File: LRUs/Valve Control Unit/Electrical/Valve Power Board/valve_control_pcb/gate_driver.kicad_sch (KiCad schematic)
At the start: 10 parts, among them U14 UCC27524D, U15 UCC27524D

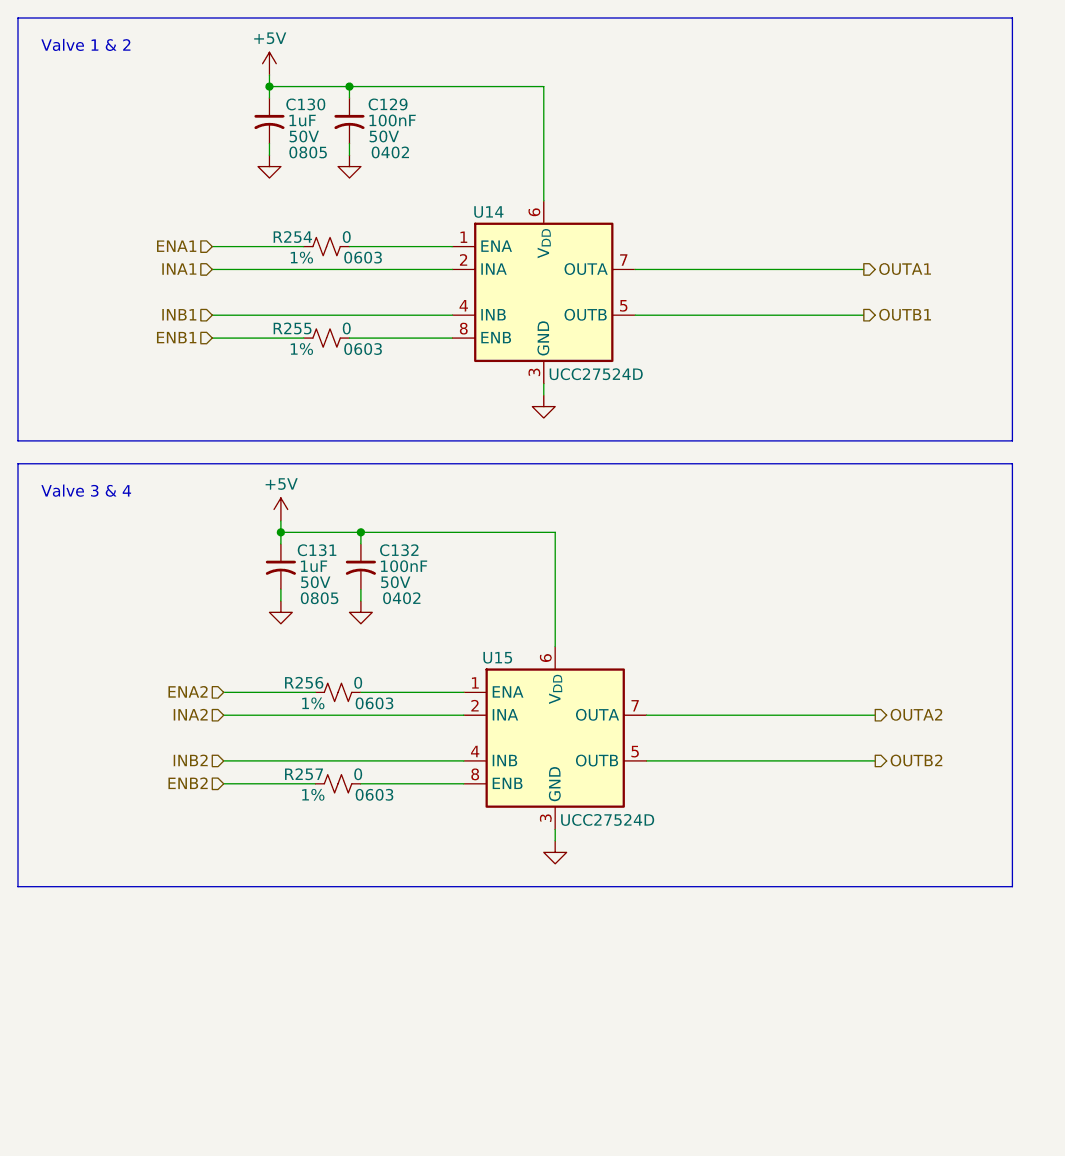
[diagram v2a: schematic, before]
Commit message: Small updates
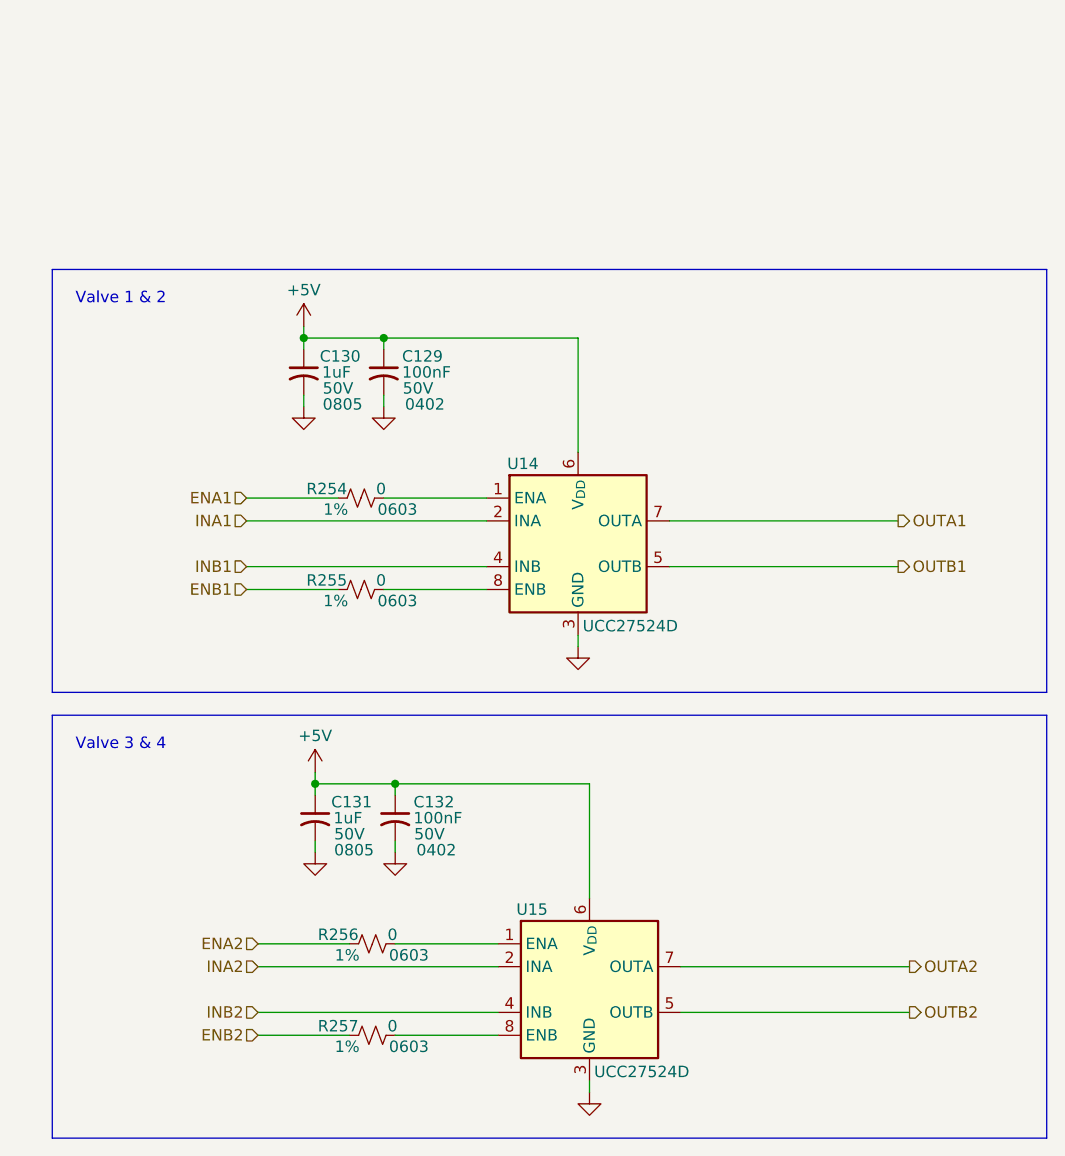
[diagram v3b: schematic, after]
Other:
- moved on the sheet: C129, C130, C131, C132, R254, R255, R256, R257, U14, U15
